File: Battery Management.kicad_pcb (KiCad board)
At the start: 2 copper layers, 33.5 x 46.6 mm, 23 parts, among them J1 Conn_01x02, J2 Conn_01x02, J3 Conn_01x02, J4 Conn_01x02, J5 Conn_01x02, Q1 PMOS, Q2 NMOS, U1 LT1996CMS_PBF, U2 ATmega328P-A, U3 MIC5219-5.0YM5, Y1 Crystal

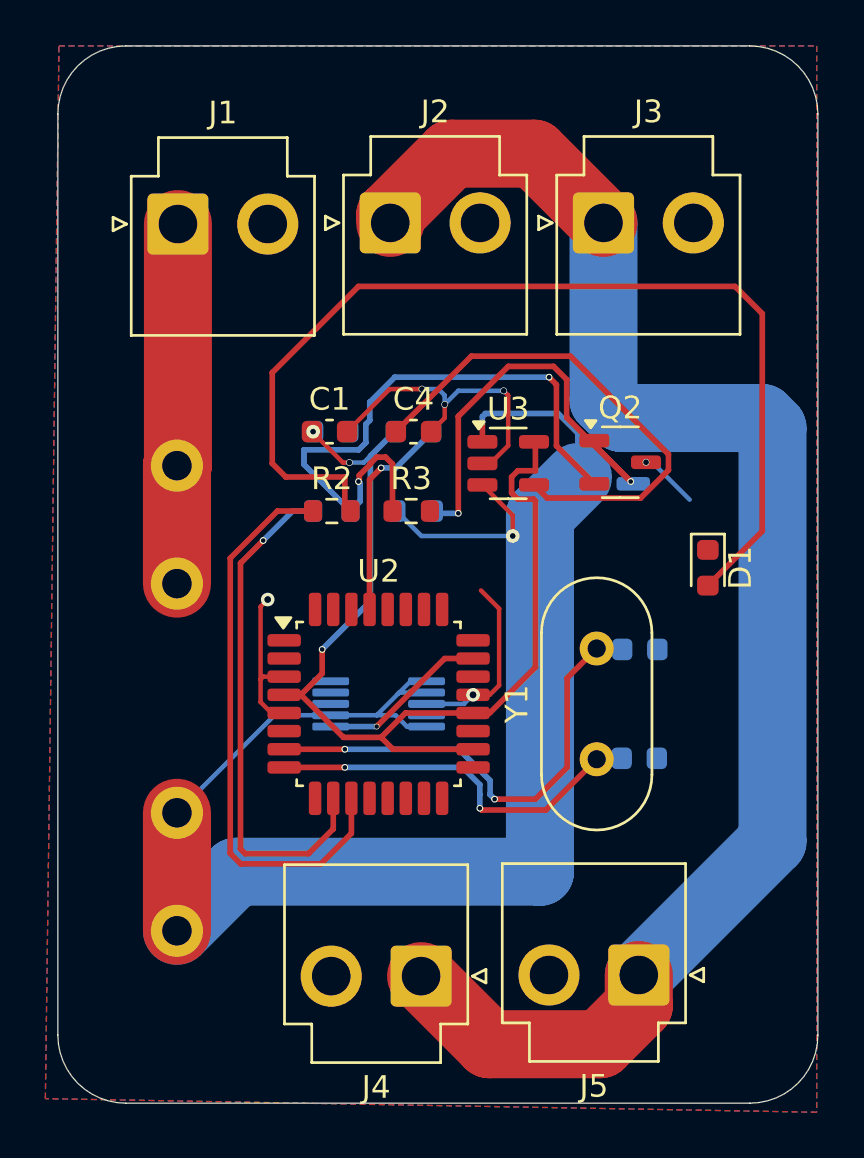
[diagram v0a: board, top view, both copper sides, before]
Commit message: Add files via upload
New battery files
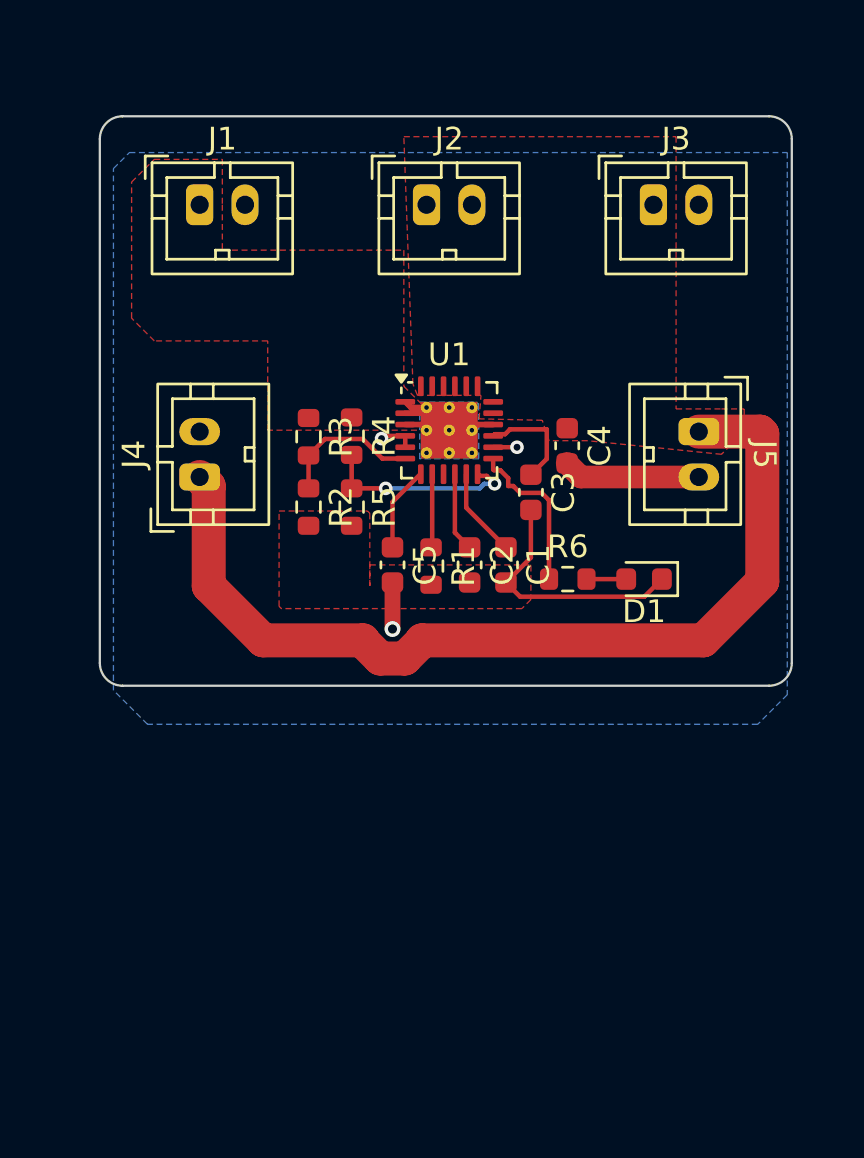
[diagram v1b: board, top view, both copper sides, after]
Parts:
- removed F1: Fuse, Fuse:Fuseholder_Littelfuse_445_030_series_5x20mm
- removed Q1: PMOS, Package_TO_SOT_SMD:SOT-23
- removed Q2: NMOS, Package_TO_SOT_SMD:SOT-23-3
- removed U2: ATmega328P-A, Package_QFP:TQFP-32_7x7mm_P0.8mm
- removed U3: MIC5219-5.0YM5, Package_TO_SOT_SMD:SOT-23-5
- removed Y1: Crystal, Crystal:Crystal_HC49-U_Vertical
- added R6: 10K, Resistor_SMD:R_0603_1608Metric, F.Cu at (96.2, 91.5)
- C1: value 0.1uF -> 330pF
- C2: value 22pF -> 128pF; moved to F.Cu
- C3: value 22pF -> 2.2nF; moved to F.Cu
- C4: value 470pF -> 470nF
- C5: value 2.2uF -> 22nF; moved to F.Cu
- J1, J2, J3, J4, J5: footprint Connector_JST:JST_VH_B2P-VH-B_1x02_P3.96mm_Vertical -> Connector_TE-Connectivity:TE_440054-2_1x02_P2.00mm_Vertical
- R1: value 10K -> 148; moved to F.Cu
- R2: value 10K -> 225k
- R3: value 10K -> 1M
- R4: value 100 -> 1M; moved to F.Cu
- R5: value 10K -> 2k; moved to F.Cu
- U1: value LT1996CMS_PBF -> TSP25983; footprint Package_SO:MSOP-10_3x3mm_P0.5mm -> Package_DFN_QFN:VQFN-24-1EP_4x4mm_P0.5mm_EP2.5x2.5mm_ThermalVias; moved to F.Cu
- moved J5 24.1 mm to (102.0, 85.0), turned to -90 degrees
- moved J4 24.1 mm to (80.0, 87.0), turned to 90 degrees
- moved C3 12.7 mm to (94.6, 87.7), turned to -90 degrees
- moved U1 12.5 mm to (91.0, 84.9), turned to 0 degrees
- moved C1 9.75 mm to (93.5, 90.9), turned to -90 degrees
- moved C2 8.37 mm to (91.9, 90.9), turned to -90 degrees
- moved C4 6.80 mm to (96.2, 85.6), turned to -90 degrees
- moved C5 6.48 mm to (88.5, 90.9), turned to -90 degrees
- moved R1 5.98 mm to (90.2, 90.9), turned to -90 degrees
- moved R3 5.59 mm to (84.8, 85.2), turned to -90 degrees
- moved R4 3.41 mm to (86.7, 85.2), turned to -90 degrees
- moved D1 2.86 mm to (99.6, 91.5), turned to 180 degrees
- moved R5 2.81 mm to (86.7, 88.3), turned to -90 degrees
- moved J3 2.34 mm to (100.0, 75.0)
- moved J2 1.79 mm to (90.0, 75.0)
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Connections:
- C1 pad 1: +5V -> Net-(U1-NRETRY)
- C2 pad 1: Net-(U2-XTAL1/PB6) -> Net-(U1-RETRY_DLY)
- C3 pad 1: Net-(U2-XTAL2/PB7) -> Net-(U1-DV/DT_BGATE)
- C4 pad 1: Net-(U3-BP) -> +6.6V
- C5 pad 1: +5V -> Net-(U1-ITIMER)
- J1 pad 1: Net-(J1-Pin_1) -> +BATT
- R1 pad 1: Net-(U2-~{RESET}/PC6) -> Net-(U1-ILIM)
- R1 pad 2: +5V -> GND
- R2 pad 1: Net-(U2-PD7) -> Net-(U1-EN/UVLO)
- R2 pad 2: Net-(D1-A) -> GND
- R3 pad 1: Net-(Q2-G) -> +BATT
- R3 pad 2: GND -> Net-(U1-EN/UVLO)
- R4 pad 1: Net-(Q2-G) -> +BATT
- R4 pad 2: Net-(U2-PD6) -> Net-(U1-OVLO)
- R5 pad 1: Net-(Q1-G) -> Net-(U1-OVLO)
- R5 pad 2: +BATT -> GND
- U1 pad 10: unconnected-(U1-M9-Pad10) -> Net-(U1-RETRY_DLY)
- U1 pad 3: GND -> +BATT
- U1 pad 5: +BATT -> GND
- U1 pad 6: VREF -> Net-(U1-EN/UVLO)
- U1 pad 7: +BATT -> Net-(U1-ITIMER)
- U1 pad 8: unconnected-(U1-M81-Pad8) -> Net-(U1-ILIM)
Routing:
- net +BATT: track 73.5 -> 5.37 mm, vias 2 -> 0
- net +5V: track 45.7 -> 0.00 mm, vias 3 -> 0
- net Net-(D1-A): track 45.7 -> 1.75 mm
- net Net-(Q2-G): track 28.0 -> 0.00 mm, vias 2 -> 0
- net +6.6V: track 67.3 -> 41.5 mm
- net Net-(U2-PD7): track 25.2 -> 0.00 mm
- net Net-(U2-PD6): track 22.7 -> 0.00 mm, vias 1 -> 0
- net Net-(U3-BP): track 22.6 -> 0.00 mm
- net Net-(U2-XTAL1/PB6): track 20.3 -> 0.00 mm, vias 2 -> 0
- net Net-(Q1-G): track 19.4 -> 0.00 mm, vias 2 -> 0
- net Net-(U2-XTAL2/PB7): track 16.1 -> 0.00 mm, vias 2 -> 0
- net Net-(J1-Pin_1): track 15.9 -> 0.00 mm
- net GND: track 31.5 -> 21.9 mm, vias 6 -> 3
- net Net-(U2-~{RESET}/PC6): track 9.36 -> 0.00 mm, vias 1 -> 0
- net Net-(U1-OVLO): track 0.00 -> 8.78 mm, vias 0 -> 2
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- added copper zone on F.Cu, net +6.6V
- added copper zone on B.Cu, net +BATT
- added copper zone on F.Cu, net +BATT
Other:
- board size 33.5 x 46.6 mm -> 30.5 x 25.1 mm
